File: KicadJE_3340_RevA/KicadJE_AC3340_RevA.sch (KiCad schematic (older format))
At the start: 125 parts, among them J101 RampOut1, J102 PulseOut2, J103 SawOut3, J104 In1.1, J105 In1.2, J106 In1.3, J107 SS_In2, J108 HS_In3, J109 FM_In4, J110 PWM_In5, J111 SineOut4, P101 HEADER_2x5_Doepfer, Q101 MMBT3906, Q102 UMX1N, SW101 Octave (3 state), U101 TL072, U102 TL072, U103 TL072, U104 AS3340, U105 L78L05_SOT89, U106 L79L05_SOT89, U107 TL072

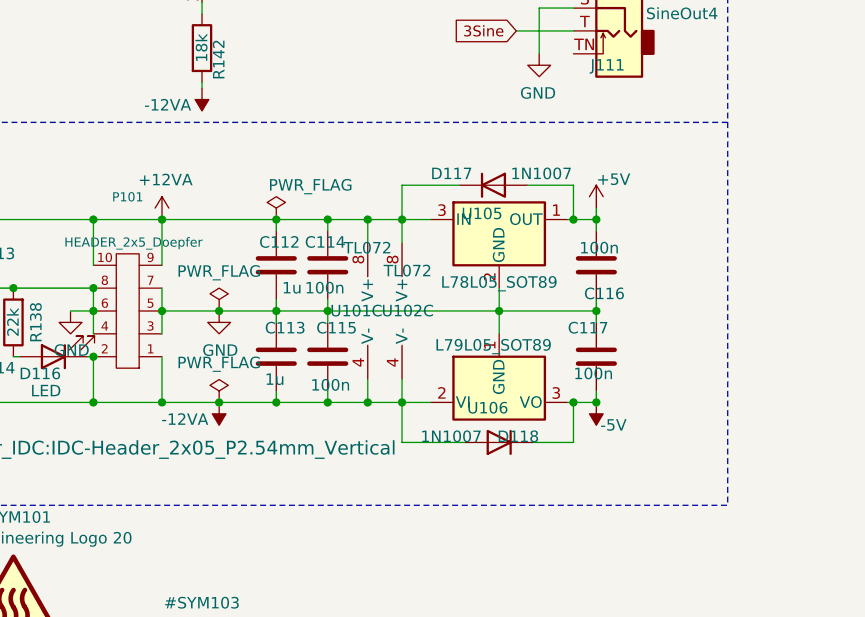
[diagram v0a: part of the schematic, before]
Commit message: DRC Done
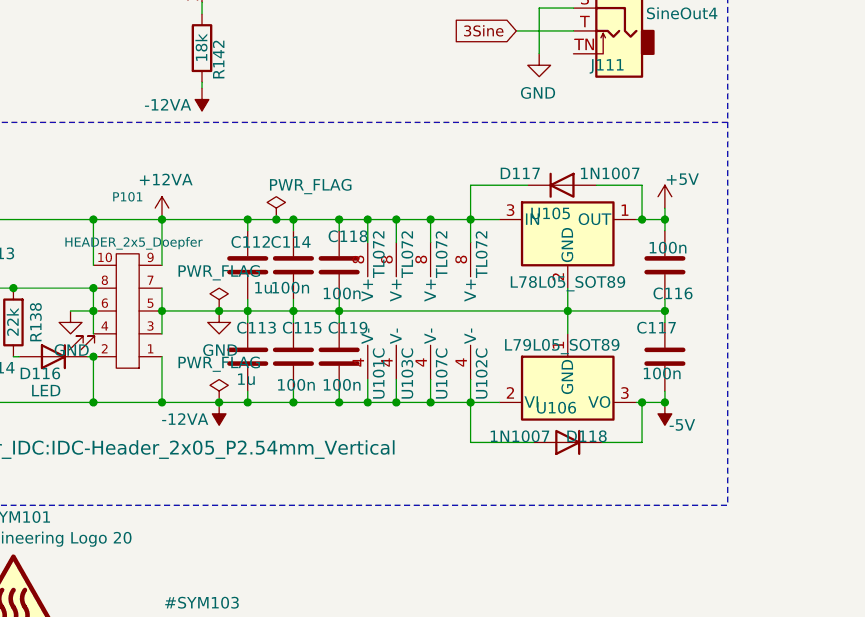
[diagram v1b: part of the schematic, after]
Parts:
- added C118, C119: 100n, Capacitor_SMD:C_0805_2012Metric_Pad1.15x1.40mm_HandSolder, symbol Device:C
- added unit 3 of U103
- added unit 3 of U107
- D115: footprint (none) -> Diode_THT:D_A-405_P7.62mm_Horizontal
- Q102: footprint UMT6 -> AJ:UMX1N_UMT6_DualNPN
- U104: footprint (none) -> Package_DIP:DIP-16_W10.16mm_LongPads
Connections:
- net +12VA: now also C118.1, U103.8 (V+), U107.8 (V+)
- net -12VA: now also C119.2, U103.4 (V-), U107.4 (V-)
- net GND: now also C118.2, C119.1
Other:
- moved on the sheet: C112, C113, C114, C115, C116, C117, D117, D118, U102C, U105, U106
